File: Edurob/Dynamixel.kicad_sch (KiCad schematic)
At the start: 5 parts, among them U2 74LVC2G241DCUTG4

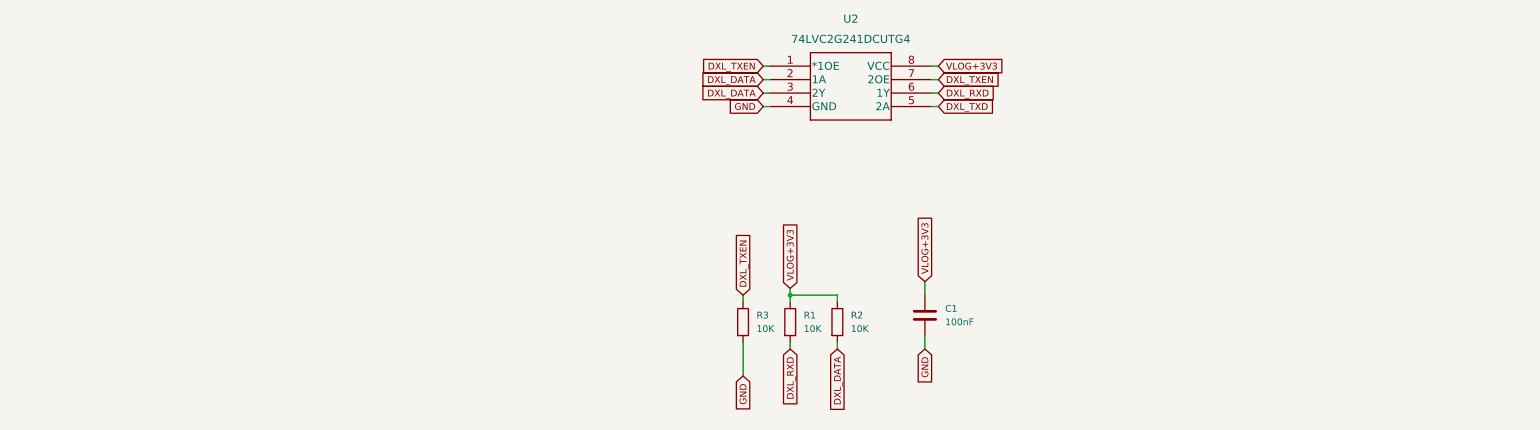
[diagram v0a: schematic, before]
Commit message: Release v1.0.1
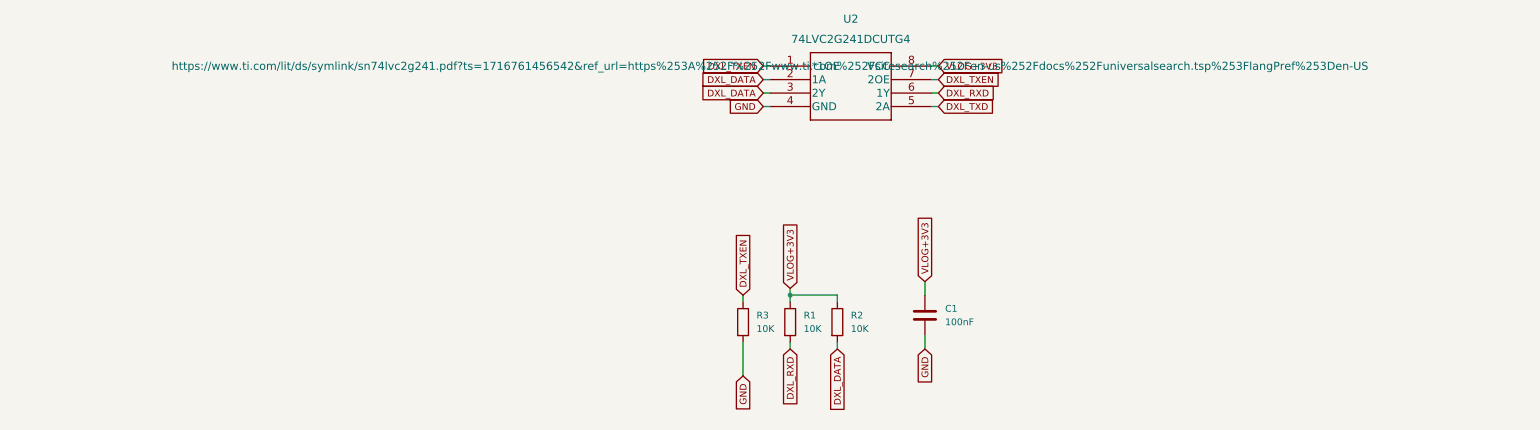
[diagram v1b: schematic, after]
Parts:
- C1: Manufacturer_Name (none) -> KYOCERA AVX; Manufacturer_Part_Number (none) -> KGM15BR71E104KT; Mouser Part Number (none) -> 581-KGM15BR71E104KT; Mouser Price/Stock (none) -> https://www.mouser.de/ProductDetail/581-KGM15BR71E104KT; Placed (none) -> True
- R1, R2, R3: Manufacturer_Name (none) -> Vishay / Dale; Manufacturer_Part_Number (none) -> CRCW060310K0FKEA; Mouser Part Number (none) -> 71-CRCW0603-10K-E3; Mouser Price/Stock (none) -> https://www.mouser.de/ProductDetail/71-CRCW0603-10K-E3; Placed (none) -> True
- U2: Manufacturer_Name (none) -> Texas Instruments; Manufacturer_Part_Number (none) -> 74LVC2G241DCUTG4; Mouser Part Number (none) -> 595-74LVC2G241DCUTG4; Mouser Price/Stock (none) -> https://www.mouser.de/ProductDetail/595-74LVC2G241DCUTG4; Placed (none) -> True
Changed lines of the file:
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@@
+      (effects (font (size 1.27 1.27)) hide)
+    )
+    (property "Manufacturer_Name" "Vishay / Dale" (at 22.86 72.39 0)
+      (effects (font (size 1.27 1.27)) hide)
+    )
+    (property "Manufacturer_Part_Number" "CRCW060310K0FKEA" (at 22.86 72.39 0)
+      (effects (font (size 1.27 1.27)) hide)
+    )
+    (property "Mouser Part Number" "71-CRCW0603-10K-E3" (at 22.86 72.39 0)
+      (effects (font (size 1.27 1.27)) hide)
+    )
+    (property "Mouser Price/Stock" "https://www.mouser.de/ProductDetail/71-CRCW0603-10K-E3" (at 22.86 72.39 0)
+      (effects (font (size 1.27 1.27)) hide)
+    )
+    (property "Placed" "True" (at 22.86 72.39 0)
       (effects (font (size 1.27 1.27)) hide)
     )
@@
       (effects (font (size 1.524 1.524)) hide)
     )
-    (property "Datasheet" "" (at 27.94 24.13 0)
+    (property "Datasheet" "https://www.ti.com/lit/ds/symlink/sn74lvc2g241.pdf?ts=1716761456542&ref_url=https%253A%252F%252Fwww.ti.com%252Fsitesearch%252Fen-us%252Fdocs%252Funiversalsearch.tsp%253FlangPref%253Den-US" (at 27.94 24.13 0)
       (effects (font (size 1.524 1.524)))
+    )
+    (property "Manufacturer_Name" "Texas Instruments" (at 43.18 27.94 0)
+      (effects (font (size 1.27 1.27)) hide)
+    )
+    (property "Manufacturer_Part_Number" "74LVC2G241DCUTG4" (at 43.18 27.94 0)
+      (effects (font (size 1.27 1.27)) hide)
+    )
+    (property "Mouser Part Number" "595-74LVC2G241DCUTG4" (at 43.18 27.94 0)
+      (effects (font (size 1.27 1.27)) hide)
+    )
+    (property "Mouser Price/Stock" "https://www.mouser.de/ProductDetail/595-74LVC2G241DCUTG4" (at 43.18 27.94 0)
+      (effects (font (size 1.27 1.27)) hide)
+    )
+    (property "Placed" "True" (at 43.18 27.94 0)
+      (effects (font (size 1.27 1.27)) hide)
     )
     (pin "1")
@@
       (effects (font (size 1.27 1.27)) hide)
     )
+    (property "Manufacturer_Name" "KYOCERA AVX" (at 57.15 71.12 0)
+      (effects (font (size 1.27 1.27)) hide)
+    )
+    (property "Manufacturer_Part_Number" "KGM15BR71E104KT" (at 57.15 71.12 0)
+      (effects (font (size 1.27 1.27)) hide)
+    )
+    (property "Mouser Part Number" "581-KGM15BR71E104KT" (at 57.15 71.12 0)
+      (effects (font (size 1.27 1.27)) hide)
+    )
+    (property "Mouser Price/Stock" "https://www.mouser.de/ProductDetail/581-KGM15BR71E104KT" (at 57.15 71.12 0)
+      (effects (font (size 1.27 1.27)) hide)
+    )
+    (property "Placed" "True" (at 57.15 71.12 0)
+      (effects (font (size 1.27 1.27)) hide)
+    )
     (pin "1")
     (pin "2")
@@
     )
     (property "Datasheet" "~" (at 31.75 72.39 0)
+      (effects (font (size 1.27 1.27)) hide)
+    )
+    (property "Manufacturer_Name" "Vishay / Dale" (at 31.75 72.39 0)
+      (effects (font (size 1.27 1.27)) hide)
+    )
+    (property "Manufacturer_Part_Number" "CRCW060310K0FKEA" (at 31.75 72.39 0)
+      (effects (font (size 1.27 1.27)) hide)
+    )
+    (property "Mouser Part Number" "71-CRCW0603-10K-E3" (at 31.75 72.39 0)
+      (effects (font (size 1.27 1.27)) hide)
+    )
+    (property "Mouser Price/Stock" "https://www.mouser.de/ProductDetail/71-CRCW0603-10K-E3" (at 31.75 72.39 0)
+      (effects (font (size 1.27 1.27)) hide)
+    )
+    (property "Placed" "True" (at 31.75 72.39 0)
       (effects (font (size 1.27 1.27)) hide)
     )
@@
       (effects (font (size 1.27 1.27)) hide)
     )
+    (property "Manufacturer_Name" "Vishay / Dale" (at 40.64 72.39 0)
+      (effects (font (size 1.27 1.27)) hide)
+    )
+    (property "Manufacturer_Part_Number" "CRCW060310K0FKEA" (at 40.64 72.39 0)
+      (effects (font (size 1.27 1.27)) hide)
+    )
+    (property "Mouser Part Number" "71-CRCW0603-10K-E3" (at 40.64 72.39 0)
+      (effects (font (size 1.27 1.27)) hide)
+    )
+    (property "Mouser Price/Stock" "https://www.mouser.de/ProductDetail/71-CRCW0603-10K-E3" (at 40.64 72.39 0)
+      (effects (font (size 1.27 1.27)) hide)
+    )
+    (property "Placed" "True" (at 40.64 72.39 0)
+      (effects (font (size 1.27 1.27)) hide)
+    )
